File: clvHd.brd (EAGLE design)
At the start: 21 x 35 mm, 41 parts, among them IC1 LMV324M, X1 009176002, X2 009176002, X3 SSW-101-02-G-S, X4 009176002, X5 SSW-101-02-G-S, X6 009176002, X7 SSW-101-02-G-S

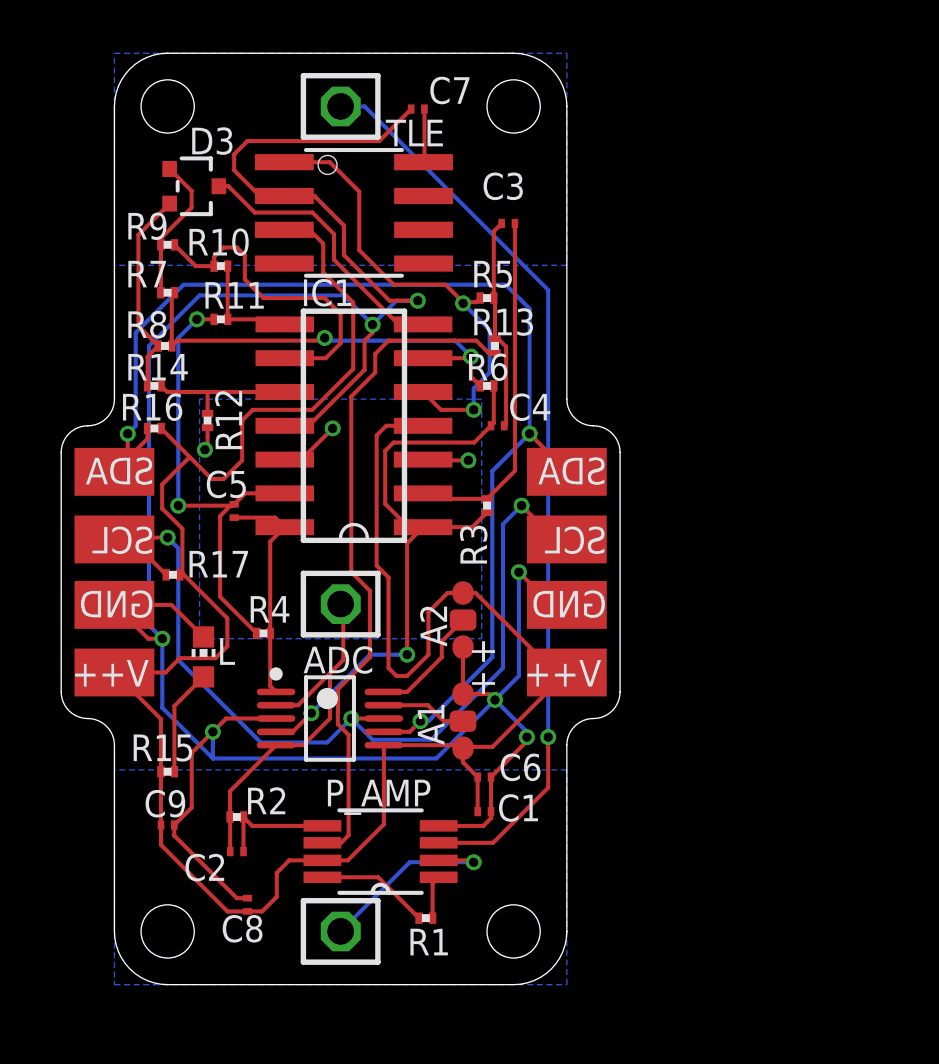
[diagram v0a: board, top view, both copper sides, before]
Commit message: update
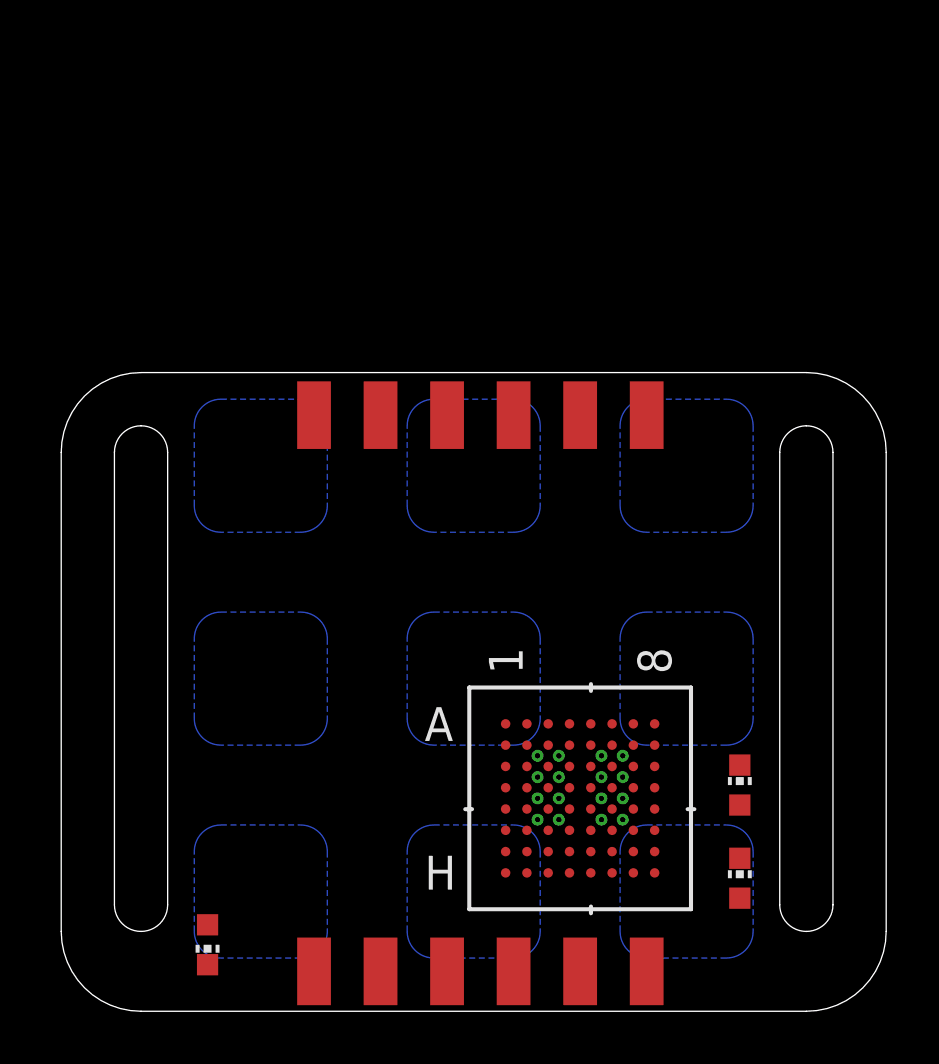
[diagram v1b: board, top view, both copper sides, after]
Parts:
- removed A1, A2: 0R-JUMPC, jump-0r-smd:C0R-JMP
- removed ADC: MICROCHIP_MCP3427-E-UNMICROCHIP_MCP3427-E-UN_0_0, UN:MICROCHIP_MCP3427-E-UN_0
- removed C1, C3, C4, C5, C6, C7, C8, C9: 0.1nF, rcl:C0201
- removed C2: 1nF, rcl:C0201
- removed D3: HSMS-285C, avago:SOT323
- removed IC1: LMV324M, linear:SO14
- removed L: (no value), led:CHIP-LED0603
- removed P_AMP: INA326EA/250, INA326EA_250:SOP65P490X110-8N
- removed R1, R10, R11, R12, R13, R14, R16, R17, R2, R3, R4, R5, R6, R7, R8, R9: 100k, rcl:R0201
- removed R15: (no value), rcl:R0201
- removed TLE: TLE2426CD, tle2426:SO-8
- removed X1, X2, X4, X6: 009176002, con-avxPerso:009176002
- removed X3, X5, X7: SSW-101-02-G-S, con-samtec:SSW-101-02-G-S
- added LED1, LED2, LED3: (no value), led:CHIP-LED0603
- added PAD1, PAD10, PAD11, PAD12, PAD2, PAD3, PAD4, PAD5, PAD6, PAD7, PAD8, PAD9: WIREPADSMD1,27-254, wirepad:SMD1,27-2,54
- added U1: ADS1298CZXGR, ADS1298ZXGR:ZXG64
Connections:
- removed net GNDA: ADC.2, ADC.5, C2.1, IC1.12, IC1.3, IC1.5, R12.1, R2.1, R5.2, TLE.1, X7.1
- removed net INM: P_AMP.2, X3.1
- removed net INP: P_AMP.3, X5.1
- removed net N$1: P_AMP.1, R1.1
- removed net N$10: IC1.6, R6.2, R7.1, R8.1
- removed net N$11: D3.2, R14.2, R8.2
- removed net N$12: IC1.9, R10.1, R9.2
- removed net N$13: D3.3, IC1.7
- removed net N$14: D3.1, R7.2, R9.1
- removed net N$15: IC1.8, R10.2, R11.1
- removed net N$16: ADC.1, C5.2, IC1.14, R4.2
- removed net N$17: ADC.7, R16.2, X2.1, X6.1
- removed net N$18: IC1.10, R12.2, R14.1
- removed net N$2: P_AMP.8, R1.2
- removed net N$23: ADC.4, C4.1, IC1.1, R3.2, R6.1
- removed net N$4: C2.2, P_AMP.5, R2.2
- removed net N$54: L.A, R15.2
- removed net N$55: C7.1, TLE.8
- removed net N$56: ADC.8, R17.2, X2.2, X6.2
- removed net N$57: A1.2, ADC.9
- removed net N$58: A2.2, ADC.10
- removed net N$6: C3.1, IC1.2, R3.1
- removed net N$7: C3.2, C4.2, R13.2, R5.1
- removed net N$8: C5.1, IC1.13, R11.2, R4.1
- removed net N$9: P_AMP.6, R13.1
- removed net V+: A1.3, A2.3, ADC.6, C1.1, C6.1, C8.2, C9.2, IC1.4, P_AMP.7, R15.1, R16.1, R17.1, TLE.3, X1.2, X4.2
- removed net V-: A1.1, A2.1, ADC.3, C1.2, C6.2, C7.2, C8.1, C9.1, IC1.11, L.C, P_AMP.4, TLE.2, X1.1, X4.1
- new net IN1: U1.H1
- new net IN2: U1.G1
- new net REF: U1.G2, U1.H2
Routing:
- net V-: track 99.1 -> 0.00 mm, vias 7 -> 0
- net V+: track 84.2 -> 0.00 mm
- net N$17: track 44.6 -> 0.00 mm, vias 3 -> 0
- net GNDA: track 36.9 -> 0.00 mm, vias 5 -> 0
- net N$56: track 34.4 -> 0.00 mm, vias 3 -> 0
- net INP: track 34.3 -> 0.00 mm, vias 1 -> 0
- net N$9: track 25.4 -> 0.00 mm, vias 0 -> 1
- net N$23: track 23.5 -> 0.00 mm, vias 2 -> 0
- net N$8: track 17.8 -> 0.00 mm, vias 2 -> 1
- net N$10: track 16.8 -> 0.00 mm, vias 2 -> 1
- net N$6: track 13.3 -> 0.00 mm, vias 0 -> 1
- net N$12: track 12.1 -> 0.00 mm, vias 0 -> 1
- net N$13: track 10.4 -> 0.00 mm, vias 0 -> 1
- net N$16: track 8.56 -> 0.00 mm, vias 0 -> 1
- net N$7: track 8.02 -> 0.00 mm, vias 0 -> 1
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- added copper zone on layer 16, net IN1
- added copper zone on layer 16, net IN3
- added copper zone on layer 16, net IN4
- added copper zone on layer 16, net IN5
- added copper zone on layer 16, net IN6
- added copper zone on layer 16, net IN7
- added copper zone on layer 16, net IN8
- added copper zone on layer 16, net IN9
- added copper zone on layer 16, net REF
- removed copper zone on layer 16, net GNDA
- removed copper zone on layer 16, net INM
- removed copper zone on layer 16, net INP
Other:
- board size 21 x 35 mm -> 31 x 24 mm
- board text removed: "+"
- board text removed: "ClvHd"
- board text removed: "E+"
- board text removed: "E-"
- board text removed: "GND"
- board text removed: "SCL"
- board text removed: "SDA"
- board text removed: "V++"
- board text removed: "v7"
